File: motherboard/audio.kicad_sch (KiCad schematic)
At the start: 29 parts, among them CN1 PJ-332A-6A (3.5mm Jack), J3 RIGHT SPEAKERS, J4 LEFT SPEAKERS, Q12 2SK3018W, U23 TPA2028D1YZFT, U25 TPA2028D1YZFT

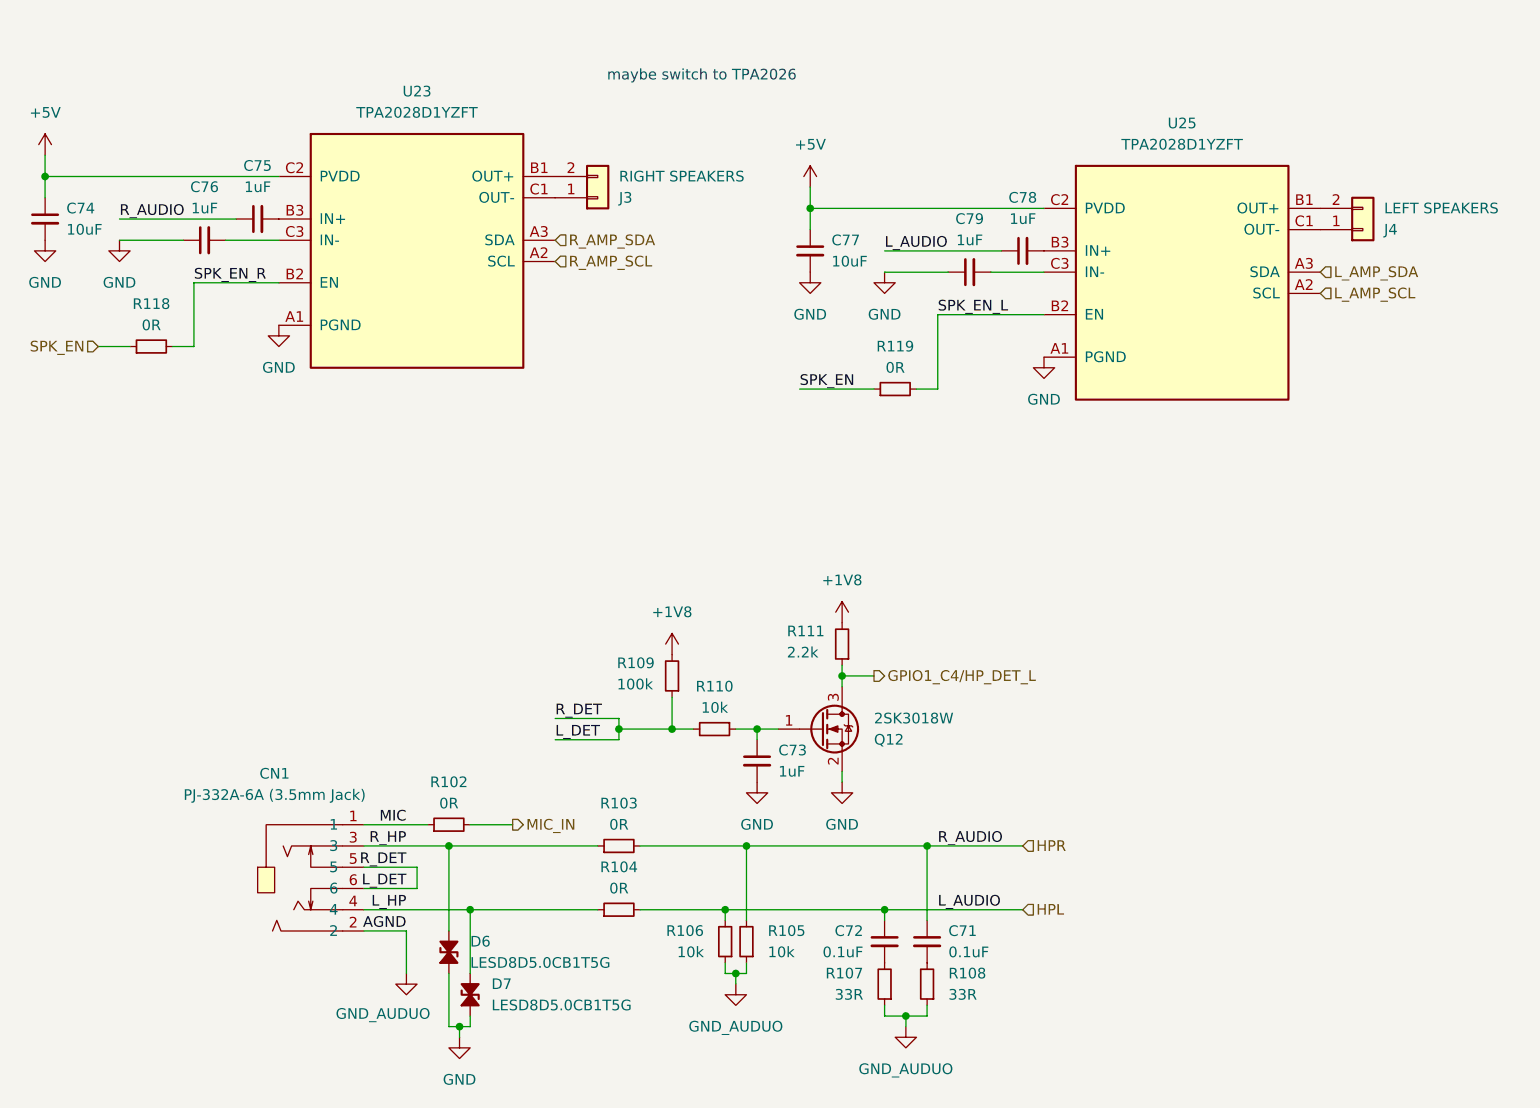
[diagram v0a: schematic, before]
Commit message: v0.2 layout
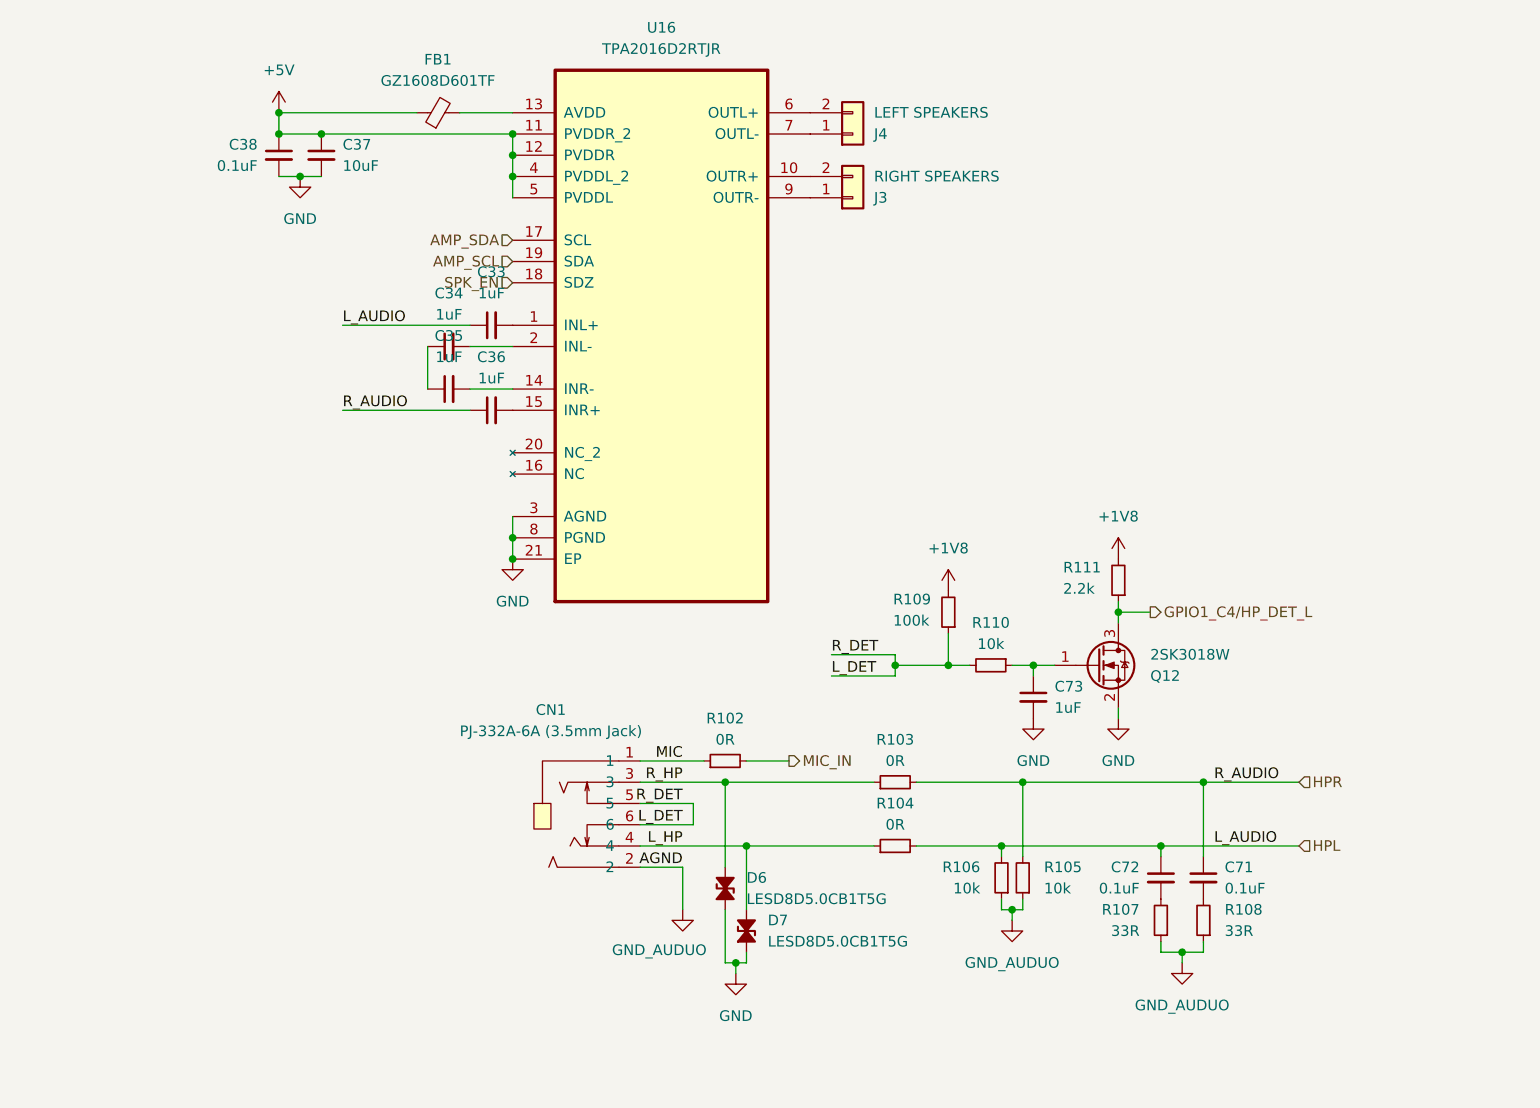
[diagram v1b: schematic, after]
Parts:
- removed C74, C77: 10uF, Capacitor_SMD:C_0603_1608Metric, symbol Device:C_Small
- removed C75, C76, C78, C79: 1uF, Capacitor_SMD:C_0402_1005Metric, symbol Device:C_Small
- removed R118, R119: 0R, Resistor_SMD:R_0402_1005Metric, symbol Device:R_Small
- removed U23, U25: TPA2028D1YZFT, Audio_Amp:BGA9C50P3X3_162X162X63, symbol Audio_Amp:TPA2028D1YZFT
- added C33, C34, C35, C36: 1uF, Capacitor_SMD:C_0402_1005Metric, symbol Device:C_Small
- added C37: 10uF, Capacitor_SMD:C_0603_1608Metric, symbol Device:C_Small
- added C38: 0.1uF, Capacitor_SMD:C_0402_1005Metric, symbol Device:C_Small
- added FB1: GZ1608D601TF, Inductor_SMD:L_0603_1608Metric, symbol Device:FerriteBead_Small
- added U16: TPA2016D2RTJR, TPA2016:QFN50P400X400X80-21N, symbol TPS2016:TPA2016D2RTJR
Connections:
- net +5V: now also C37.1, C38.1, FB1.1, U16.11 (PVDDR_2), U16.12 (PVDDR), U16.4 (PVDDL_2), U16.5 (PVDDL)
- net GND: now also C37.2, C38.2, U16.21 (EP), U16.3 (AGND), U16.8 (PGND)
- net HPL: now also C33.1
- net HPR: now also C36.1
- net SPK_EN: now also U16.18 (SDZ)
- net at J3.1 (Pin_1): now also U16.9 (OUTR-)
- net at J3.2 (Pin_2): now also U16.10 (OUTR+)
- net at J4.2 (Pin_2): now also U16.6 (OUTL+)
- net at J4.1 (Pin_1): now also U16.7 (OUTL-)
- new net: C34.1, C35.1
- new net: C35.2, U16.14 (INR-)
- new net: C33.2, U16.1 (INL+)
- new net: FB1.2, U16.13 (AVDD)
- new net: C36.2, U16.15 (INR+)
- new net: C34.2, U16.2 (INL-)
- new net AMP_SCL: U16.19 (SDA)
- new net AMP_SDA: U16.17 (SCL)
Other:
- note removed: "maybe switch to TPA2026"
- moved on the sheet: C71, C72, C73, CN1, D6, D7, J3, J4, Q12, R102, R103, R104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
